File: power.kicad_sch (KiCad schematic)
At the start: 92 parts, among them SW1 SW_Push, U26 RK806S-5

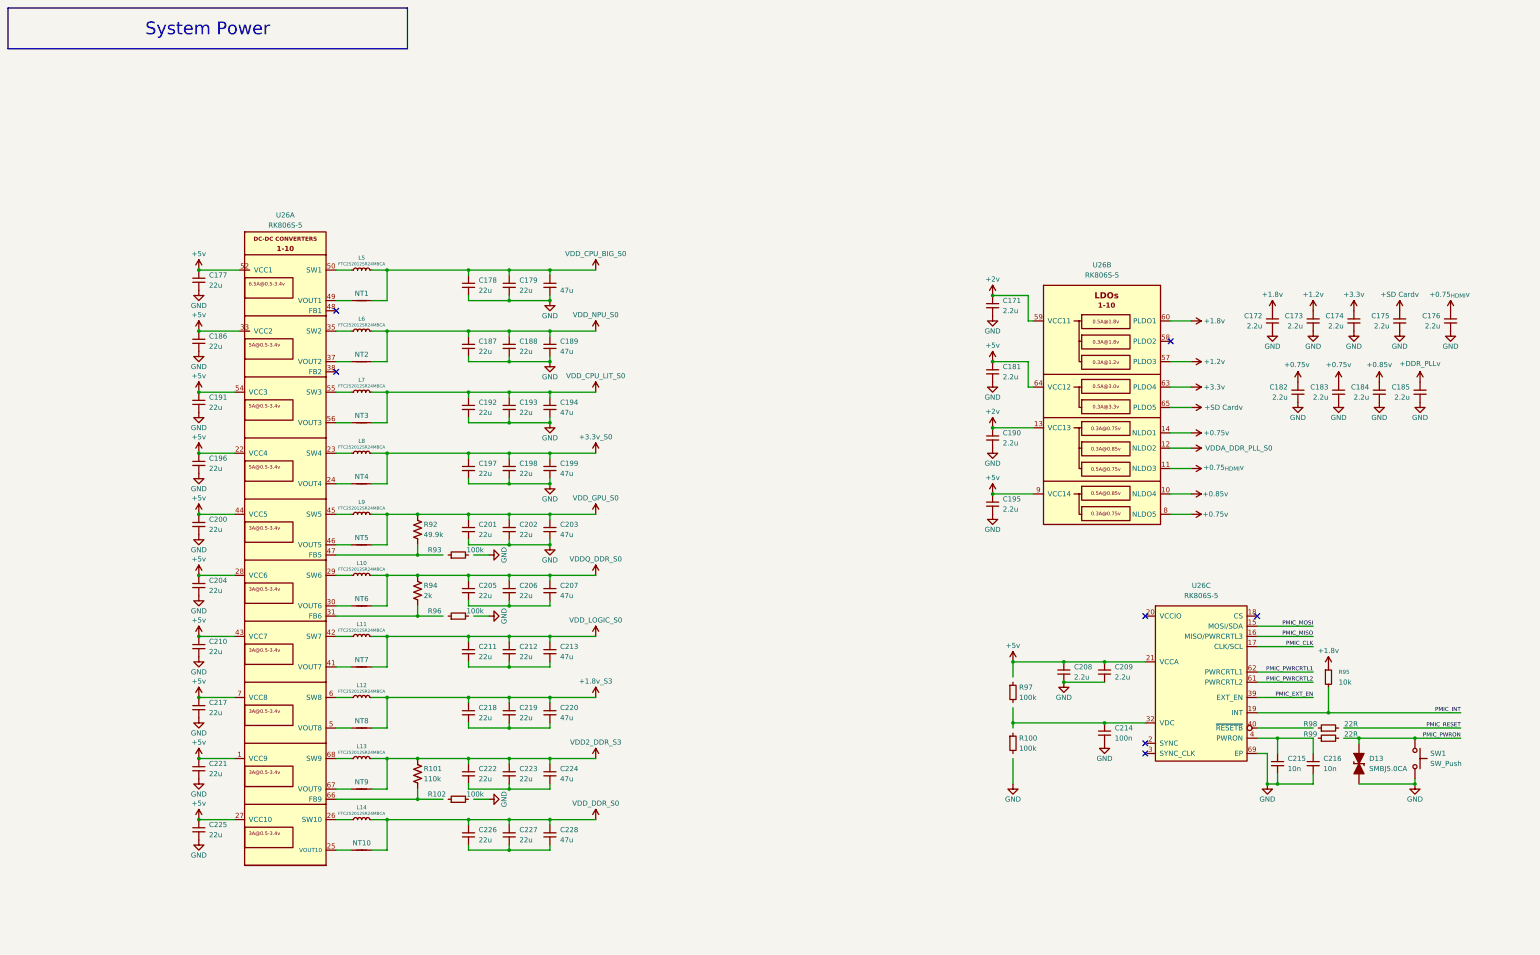
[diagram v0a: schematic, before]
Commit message: Add files via upload
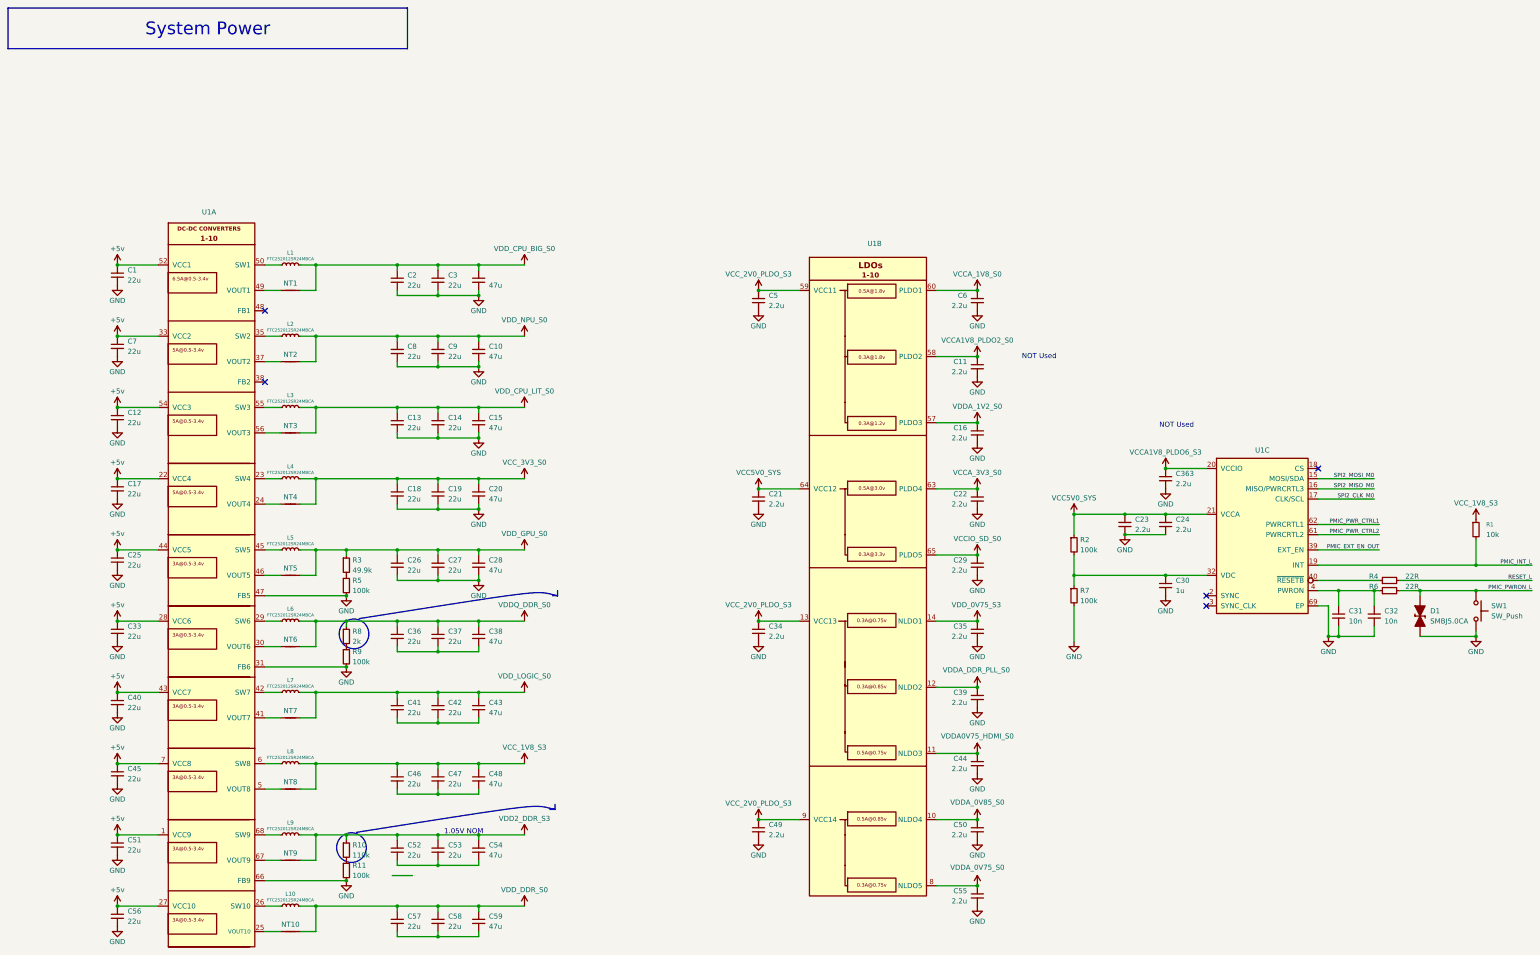
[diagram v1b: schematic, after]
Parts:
- removed C173, C174: 2.2u, Capacitor_SMD:C_0402_1005Metric, symbol New_Library_0:C_Small_edited
- removed C226, C227: 22u, Capacitor_SMD:C_0603_1608Metric, symbol New_Library_0:C_Small_edited
- removed C228: 47u, Capacitor_SMD:C_0805_2012Metric, symbol New_Library_0:C_Small_edited
- removed L14: FTC252012SR24MBCA, Inductor_SMD:L_1008_2520Metric, symbol Device:L_Small
- removed R102, R93, R96: 100k, PCM_Resistor_SMD_AKL:R_0402_1005Metric, symbol Device:R_Small
- added C11, C16, C22, C363: 2.2u, Capacitor_SMD:C_0402_1005Metric, symbol New_Library_0:C_Small_edited
- added C57, C58: 22u, Capacitor_SMD:C_0603_1608Metric, symbol New_Library_0:C_Small_edited
- added C59: 47u, Capacitor_SMD:C_0805_2012Metric, symbol New_Library_0:C_Small_edited
- added L10: FTC252012SR24MBCA, Inductor_SMD:L_1008_2520Metric, symbol Device:L_Small
- added R11, R5, R9: 100k, PCM_Resistor_SMD_AKL:R_0402_1005Metric, symbol Device:R_Small
- C30: renamed from C214; value 100n -> 1u
- R10: renamed from R101; symbol Device:R_US -> Device:R_Small
- R3: renamed from R92; symbol Device:R_US -> Device:R_Small
- R8: renamed from R94; symbol Device:R_US -> Device:R_Small
- renumbered C177 to C1, C189 to C10, C191 to C12, C192 to C13, C193 to C14, C194 to C15, C196 to C17, C197 to C18, C198 to C19, C178 to C2, C199 to C20, C181 to C21, C208 to C23, C209 to C24, C200 to C25, C201 to C26, C202 to C27, C203 to C28, C175 to C29, C179 to C3, C215 to C31, C216 to C32, C204 to C33, C190 to C34, C176 to C35, C205 to C36, C206 to C37, C207 to C38, C182 to C39, C180 to C4, C210 to C40, C211 to C41, C212 to C42, C213 to C43, C183 to C44, C217 to C45, C218 to C46, C219 to C47, C220 to C48, C195 to C49, C171 to C5, C184 to C50, C221 to C51, C222 to C52, C223 to C53, C224 to C54, C185 to C55, C225 to C56, C172 to C6, C186 to C7, C187 to C8, C188 to C9, D13 to D1, L5 to L1, L6 to L2, L7 to L3, L8 to L4, L9 to L5, L10 to L6, L11 to L7, L12 to L8, L13 to L9, R95 to R1, R97 to R2, R98 to R4, R99 to R6, R100 to R7, U26 to U1
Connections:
- net PMIC_PWRON is gone; now on net PMIC_PWRON_L: D1.2 (A), SW1.1
- net +5v: no longer C21.1, C23.1, C24.1, C49.1, U1.21 (VCCA), U1.64 (VCC12), U1.9 (VCC14)
- net GND: now also R7.2, U1.31 (FB6), U1.47 (FB5), U1.66 (FB9), C11.2, C16.2, C22.2, C363.2, R11.2, R5.2, R9.2
- net VDDA_DDR_PLL_S0: now also C39.1
- net VDD_DDR_S0: now also C57.1, C58.1, C59.1, L10.2
- net at R6.1: now also C31.1, C32.1, U1.4 (PWRON)
- net PMIC_PWRON_L: now reaches R6.2
- net at R8.2: now also R9.1; no longer U1.31 (FB6)
- net VCCA1V8_PLDO2_S0: now reaches U1.58 (PLDO2)
- net VCCA1V8_PLDO2_S0: now also C11.1
- net at U1.26 (SW10): now also L10.1
- net VCCA1V8_PLDO6_S3: now reaches U1.20 (VCCIO)
- net VCCA1V8_PLDO6_S3: now also C363.1
- net at C30.1, U1.32 (VDC): now also R2.2, R7.1
- net at U1.40 (~{RESETB}): now also R4.1
- net RESET_L: now reaches R4.2
- net VCC5V0_SYS: now reaches R2.1
- net VCC5V0_SYS: now also C21.1, C23.1, C24.1, U1.21 (VCCA), U1.64 (VCC12)
- net at R3.2: now also R5.1; no longer U1.47 (FB5)
- net at R10.2: now also R11.1; no longer U1.66 (FB9)
- net +0.75_{HDMI}v renamed VDDA0V75_HDMI_S0
- net VDDA0V75_HDMI_S0: now also C44.1; no longer C35.1
- removed net +0.75v: C39.1, C44.1, U1.14 (NLDO1), U1.8 (NLDO5)
- net +0.85v renamed VDDA_0V85_S0
- net +1.2v renamed VDDA_1V2_S0
- net VDDA_1V2_S0: now also C16.1
- net +1.8v renamed VCCA_1V8_S0
- net VCCA_1V8_S0: no longer R1.1
- net +1.8v_S3 renamed VCC_1V8_S3
- net VCC_1V8_S3: now also R1.1
- net +2v renamed VCC_2V0_PLDO_S3
- net VCC_2V0_PLDO_S3: now also C49.1, U1.9 (VCC14)
- net +3.3v renamed VCCA_3V3_S0
- net VCCA_3V3_S0: now also C22.1
- net +3.3v_S0 renamed VCC_3V3_S0
- net +DDR_PLLv renamed VDDA_0V75_S0
- net VDDA_0V75_S0: now also U1.8 (NLDO5)
- net +SD Cardv renamed VCCIO_SD_S0
- net PMIC_CLK renamed SPI2_CLK_M0
- net PMIC_EXT_EN renamed PMIC_EXT_EN_OUT
- net PMIC_INT renamed PMIC_INT_L
- net PMIC_MISO renamed SPI2_MISO_M0
- net PMIC_MOSI renamed SPI2_MOSI_M0
- net PMIC_PWRCRTL1 renamed PMIC_PWR_CTRL1
- net PMIC_PWRCRTL2 renamed PMIC_PWR_CTRL2
- new net: C57.2, C58.2, C59.2
- new net VDD_0V75_S3: C35.1, U1.14 (NLDO1)
- no-connect marks 7 -> 5
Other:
- note added: "1.05V NOM"
- moved on the sheet: C1, C10, C12, C13, C14, C15, C17, C18, C19, C2, C20, C21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
